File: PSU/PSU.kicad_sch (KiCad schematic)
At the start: 60 parts, among them J1 VBATIN, J3 12VOUT, J5 5VOUT, SW1 SW_SPST, U1 STPS10L25G-TR, U2 STPS10L25G-TR, U3 L4975A, U4 STPS10L25G-TR, U5 STPS10L25G-TR, U6 L4975A

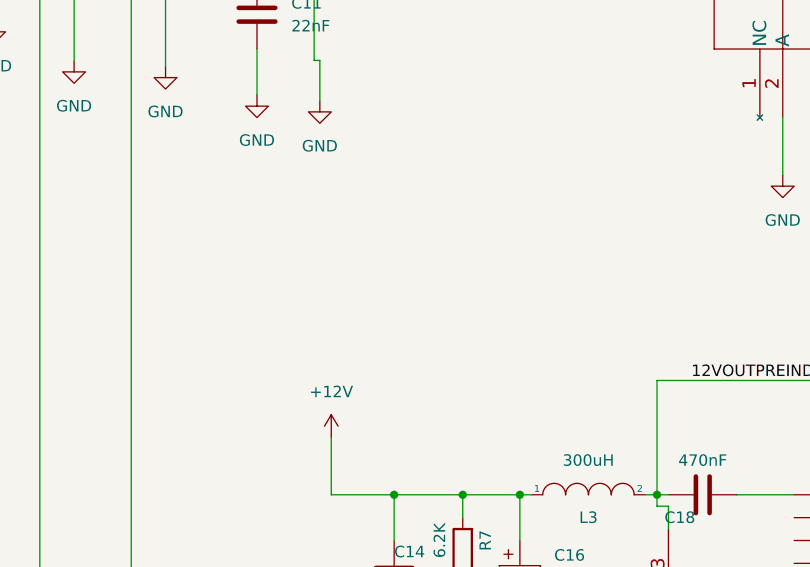
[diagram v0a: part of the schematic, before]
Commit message: Final layout
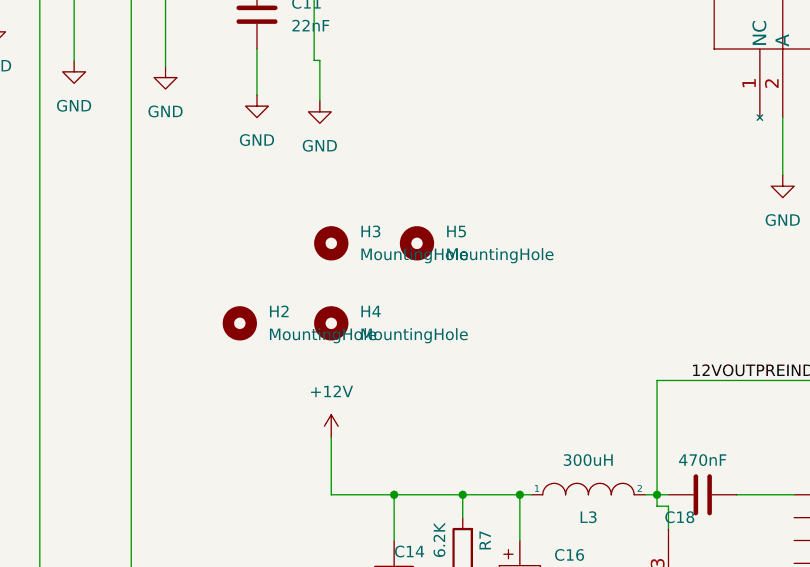
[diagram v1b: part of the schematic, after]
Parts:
- added H2, H3, H4, H5: MountingHole, MountingHole:MountingHole_3.2mm_M3, symbol Mechanical:MountingHole
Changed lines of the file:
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@@
     (pin "1")
+  )
+  (symbol (lib_id "Mechanical:MountingHole") (at 146.685 86.36 0) (unit 1)
+    (in_bom yes) (on_board yes) (fields_autoplaced)
+    (property "Reference" "H2" (id 0) (at 149.86 85.0899 0)
+      (effects (font (size 1.27 1.27)) (justify left))
+    )
+    (property "Value" "MountingHole" (id 1) (at 149.86 87.6299 0)
+      (effects (font (size 1.27 1.27)) (justify left))
+    )
+    (property "Footprint" "MountingHole:MountingHole_3.2mm_M3" (id 2) (at 146.685 86.36 0)
+      (effects (font (size 1.27 1.27)) hide)
+    )
+    (property "Datasheet" "~" (id 3) (at 146.685 86.36 0)
+      (effects (font (size 1.27 1.27)) hide)
+    )
   )
   (symbol (lib_id "Device:R") (at 201.93 -8.89 90) (unit 1)
@@
     (pin "2")
   )
+  (symbol (lib_id "Mechanical:MountingHole") (at 166.37 77.47 0) (unit 1)
+    (in_bom yes) (on_board yes) (fields_autoplaced)
+    (property "Reference" "H5" (id 0) (at 169.545 76.1999 0)
+      (effects (font (size 1.27 1.27)) (justify left))
+    )
+    (property "Value" "MountingHole" (id 1) (at 169.545 78.7399 0)
+      (effects (font (size 1.27 1.27)) (justify left))
+    )
+    (property "Footprint" "MountingHole:MountingHole_3.2mm_M3" (id 2) (at 166.37 77.47 0)
+      (effects (font (size 1.27 1.27)) hide)
+    )
+    (property "Datasheet" "~" (id 3) (at 166.37 77.47 0)
+      (effects (font (size 1.27 1.27)) hide)
+    )
+  )
   (symbol (lib_id "power:GND") (at 86.36 70.485 0) (unit 1)
     (in_bom yes) (on_board yes) (fields_autoplaced)
@@
     )
     (pin "1")
+  )
+  (symbol (lib_id "Mechanical:MountingHole") (at 156.845 86.36 0) (unit 1)
+    (in_bom yes) (on_board yes) (fields_autoplaced)
+    (property "Reference" "H4" (id 0) (at 160.02 85.0899 0)
+      (effects (font (size 1.27 1.27)) (justify left))
+    )
+    (property "Value" "MountingHole" (id 1) (at 160.02 87.6299 0)
+      (effects (font (size 1.27 1.27)) (justify left))
+    )
+    (property "Footprint" "MountingHole:MountingHole_3.2mm_M3" (id 2) (at 156.845 86.36 0)
+      (effects (font (size 1.27 1.27)) hide)
+    )
+    (property "Datasheet" "~" (id 3) (at 156.845 86.36 0)
+      (effects (font (size 1.27 1.27)) hide)
+    )
   )
   (symbol (lib_id "power:PWR_FLAG") (at 36.195 66.675 180) (unit 1)
@@
     (pin "1")
     (pin "2")
+  )
+  (symbol (lib_id "Mechanical:MountingHole") (at 156.845 77.47 0) (unit 1)
+    (in_bom yes) (on_board yes) (fields_autoplaced)
+    (property "Reference" "H3" (id 0) (at 160.02 76.1999 0)
+      (effects (font (size 1.27 1.27)) (justify left))
+    )
+    (property "Value" "MountingHole" (id 1) (at 160.02 78.7399 0)
+      (effects (font (size 1.27 1.27)) (justify left))
+    )
+    (property "Footprint" "MountingHole:MountingHole_3.2mm_M3" (id 2) (at 156.845 77.47 0)
+      (effects (font (size 1.27 1.27)) hide)
+    )
+    (property "Datasheet" "~" (id 3) (at 156.845 77.47 0)
+      (effects (font (size 1.27 1.27)) hide)
+    )
   )
   (symbol (lib_id "Device:C_Polarized") (at 177.8 114.3 0) (unit 1)
@@
       (reference "F1") (unit 1) (value "Fuse") (footprint "Fuse:Fuseholder_Littelfuse_445_030_series_5x20mm")
     )
+    (path "/26c9a61b-49de-43ad-b3c9-7b4385b6b4c9"
+      (reference "H2") (unit 1) (value "MountingHole") (footprint "MountingHole:MountingHole_3.2mm_M3")
+    )
+    (path "/7b5b1218-cc4e-45ff-8792-a3c583c7a8f3"
+      (reference "H3") (unit 1) (value "MountingHole") (footprint "MountingHole:MountingHole_3.2mm_M3")
+    )
+    (path "/5d760dc9-a87e-41f6-9335-879c04b18949"
+      (reference "H4") (unit 1) (value "MountingHole") (footprint "MountingHole:MountingHole_3.2mm_M3")
+    )
+    (path "/356c0127-d996-4c58-b7c5-ab3b4fb89928"
+      (reference "H5") (unit 1) (value "MountingHole") (footprint "MountingHole:MountingHole_3.2mm_M3")
+    )
     (path "/a0748573-0159-4f0a-9e05-0f57d7155c8e"
